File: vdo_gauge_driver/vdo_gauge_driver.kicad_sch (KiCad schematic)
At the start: 15 parts, among them J1 12V and GND, J2 12V / Signal / GND, J3 ECU Input, Q1 2N7000, SW1 SW_SPDT, U1 L7805, U3 MCP6002-xP, U4 ATtiny85-20P

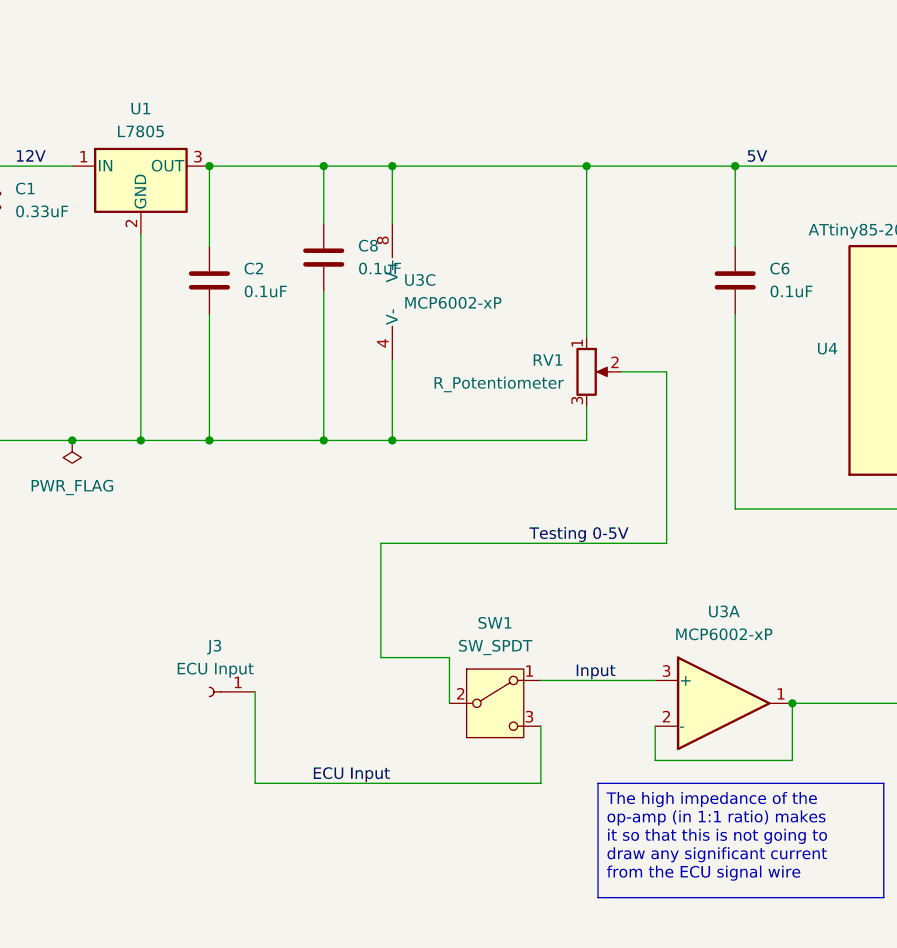
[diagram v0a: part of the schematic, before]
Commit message: Working, but unstable
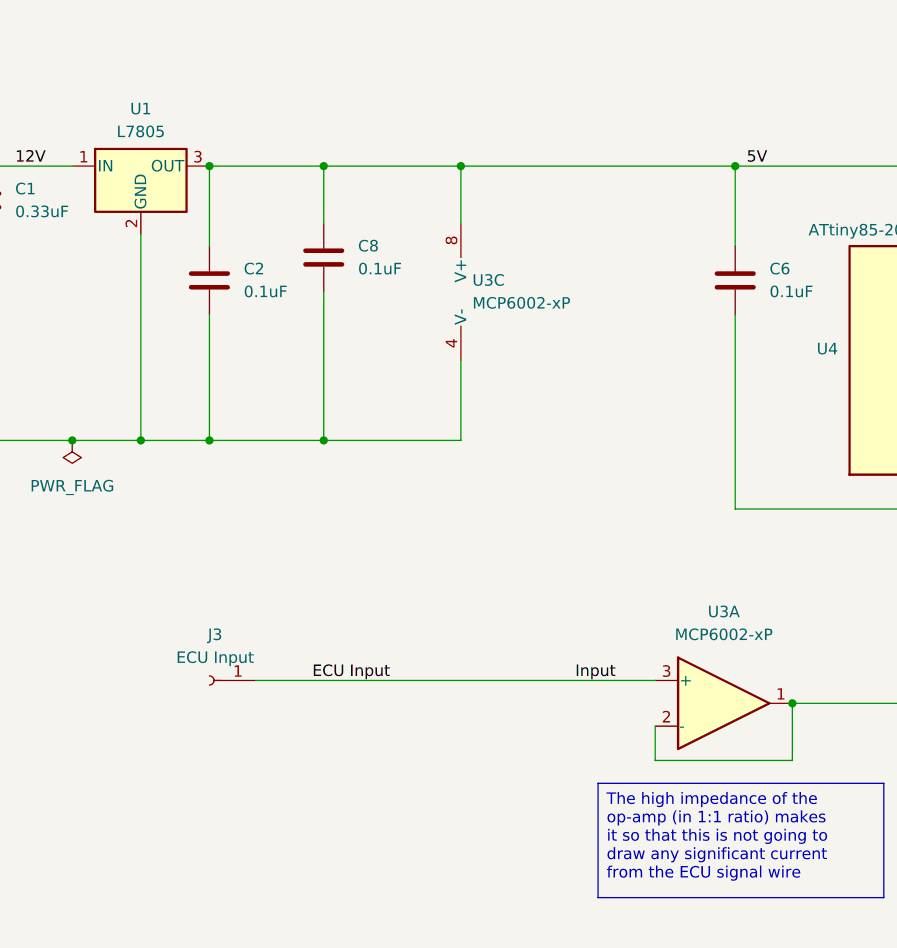
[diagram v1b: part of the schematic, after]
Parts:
- removed RV1: R_Potentiometer, Potentiometer_THT:Potentiometer_Bourns_3386P_Vertical, symbol Device:R_Potentiometer
- removed SW1: SW_SPDT, Button_Switch_THT:SW_Slide-03_Wuerth-WS-SLTV_10x2.5x6.4_P2.54mm, symbol Switch:SW_SPDT
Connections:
- net Input is gone; now on net ECU Input: U3.3 (+)
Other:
- moved on the sheet: J3, U3C
